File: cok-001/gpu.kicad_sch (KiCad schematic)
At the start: 9 parts

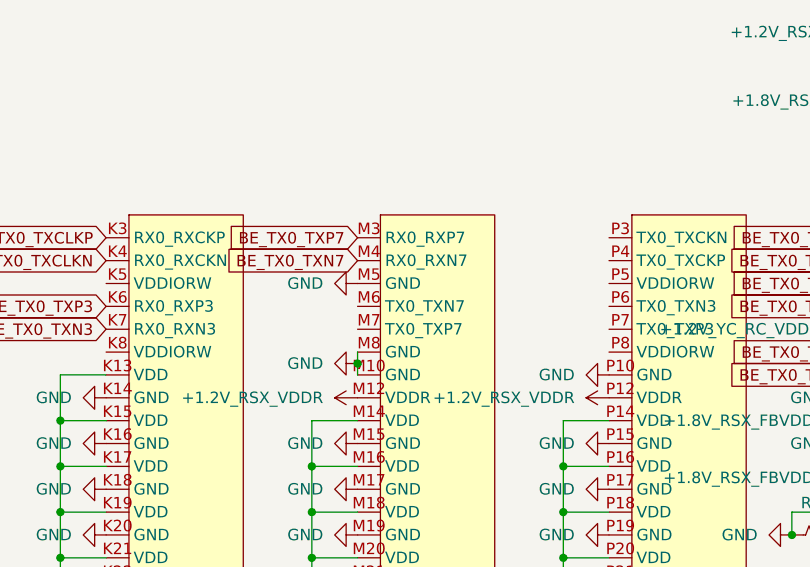
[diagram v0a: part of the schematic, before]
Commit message: ram lines
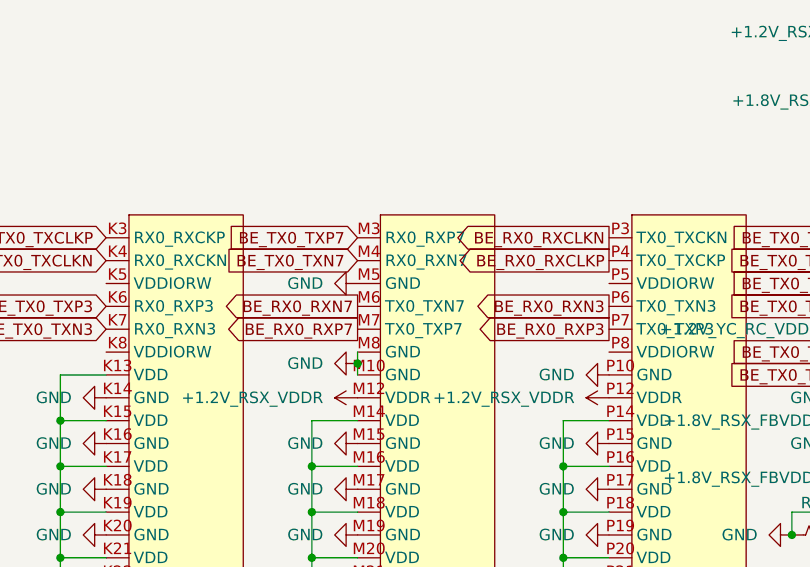
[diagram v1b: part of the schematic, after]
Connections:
- net BE_RX0_RXCLKN: now reaches U2001.P3 (TX0_TXCKN)
- net BE_RX0_RXCLKP: now reaches U2001.P4 (TX0_TXCKP)
- net BE_RX0_RXN3: now reaches U2001.P6 (TX0_TXN3)
- net BE_RX0_RXP3: now reaches U2001.P7 (TX0_TXP3)
- net BE_RX0_RXN7: now reaches U2001.M6 (TX0_TXN7)
- net BE_RX0_RXP7: now reaches U2001.M7 (TX0_TXP7)
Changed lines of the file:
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@@
+		)
+	)
+	(global_label "BE_RX0_RXP3"
+		(shape output)
+		(at 325.12 27.94 180)
+		(fields_autoplaced yes)
+		(effects
+			(font
+				(size 1.27 1.27)
+			)
+			(justify right)
+		)
+		(property "Intersheetrefs" "${INTERSHEET_REFS}"
+			(at 309.1326 27.94 0)
+			(effects
+				(font
+					(size 1.27 1.27)
+				)
+				(justify right)
+				(hide yes)
+			)
 		)
 	)
@@
 		)
 	)
+	(global_label "BE_RX0_RXN7"
+		(shape output)
+		(at 297.18 25.4 180)
+		(fields_autoplaced yes)
+		(effects
+			(font
+				(size 1.27 1.27)
+			)
+			(justify right)
+		)
+		(property "Intersheetrefs" "${INTERSHEET_REFS}"
+			(at 281.1321 25.4 0)
+			(effects
+				(font
+					(size 1.27 1.27)
+				)
+				(justify right)
+				(hide yes)
+			)
+		)
+	)
 	(global_label "BE_RX0_RXN2"
 		(shape output)
@@
 		)
 	)
+	(global_label "BE_RX0_RXN3"
+		(shape output)
+		(at 325.12 25.4 180)
+		(fields_autoplaced yes)
+		(effects
+			(font
+				(size 1.27 1.27)
+			)
+			(justify right)
+		)
+		(property "Intersheetrefs" "${INTERSHEET_REFS}"
+			(at 309.0721 25.4 0)
+			(effects
+				(font
+					(size 1.27 1.27)
+				)
+				(justify right)
+				(hide yes)
+			)
+		)
+	)
 	(global_label "RSX_VI28"
 		(shape input)
@@
 		)
 	)
+	(global_label "BE_RX0_RXCLKN"
+		(shape output)
+		(at 325.12 17.78 180)
+		(fields_autoplaced yes)
+		(effects
+			(font
+				(size 1.27 1.27)
+			)
+			(justify right)
+		)
+		(property "Intersheetrefs" "${INTERSHEET_REFS}"
+			(at 306.7135 17.78 0)
+			(effects
+				(font
+					(size 1.27 1.27)
+				)
+				(justify right)
+				(hide yes)
+			)
+		)
+	)
 	(global_label "BE_TX2_TXN6"
 		(shape input)
@@
 		)
 	)
+	(global_label "BE_RX0_RXCLKP"
+		(shape output)
+		(at 325.12 20.32 180)
+		(fields_autoplaced yes)
+		(effects
+			(font
+				(size 1.27 1.27)
+			)
+			(justify right)
+		)
+		(property "Intersheetrefs" "${INTERSHEET_REFS}"
+			(at 306.774 20.32 0)
+			(effects
+				(font
+					(size 1.27 1.27)
+				)
+				(justify right)
+				(hide yes)
+			)
+		)
+	)
 	(global_label "RSX_VO69"
 		(shape input)
@@
 			(effects
 				(font
+					(size 1.27 1.27)
+				)
+				(justify right)
+				(hide yes)
+			)
+		)
+	)
+	(global_label "BE_RX0_RXP7"
+		(shape output)
+		(at 297.18 27.94 180)
+		(fields_autoplaced yes)
+		(effects
+			(font
+				(size 1.27 1.27)
+			)
+			(justify right)
+		)
+		(property "Intersheetrefs" "${INTERSHEET_REFS}"
+			(at 281.1926 27.94 0)
+			(effects
+				(font
